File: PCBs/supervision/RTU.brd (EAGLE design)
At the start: 75 x 59 mm, 18 parts, among them IC1 LM1117T-1.8, IC2 7805T, M1 WIRELESS-NRF24L01, Q1 BC548, U1 ESP-WROOM-32, U2 MICROSD_CATALEX, U3 DS1307Z, Y2 32kHz

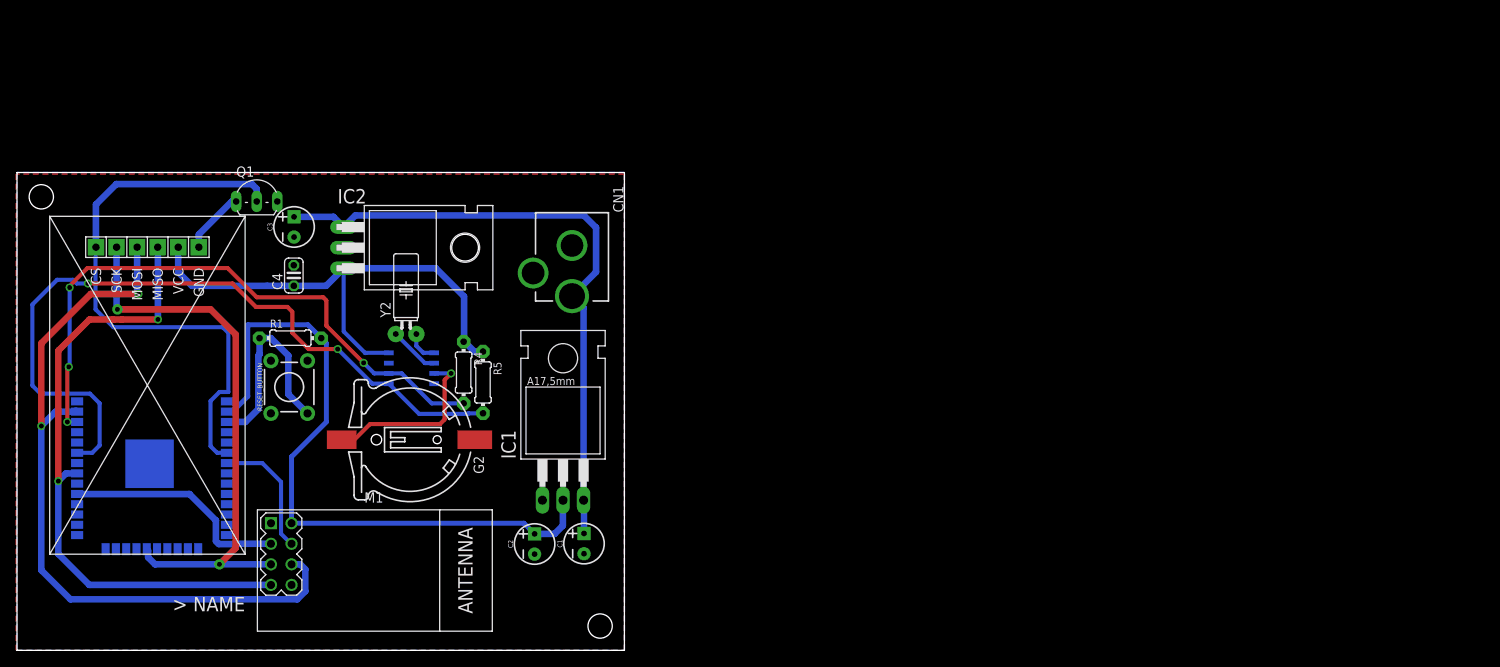
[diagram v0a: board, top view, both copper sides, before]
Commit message: Re-prototipação da PCB do sistema supervisorio
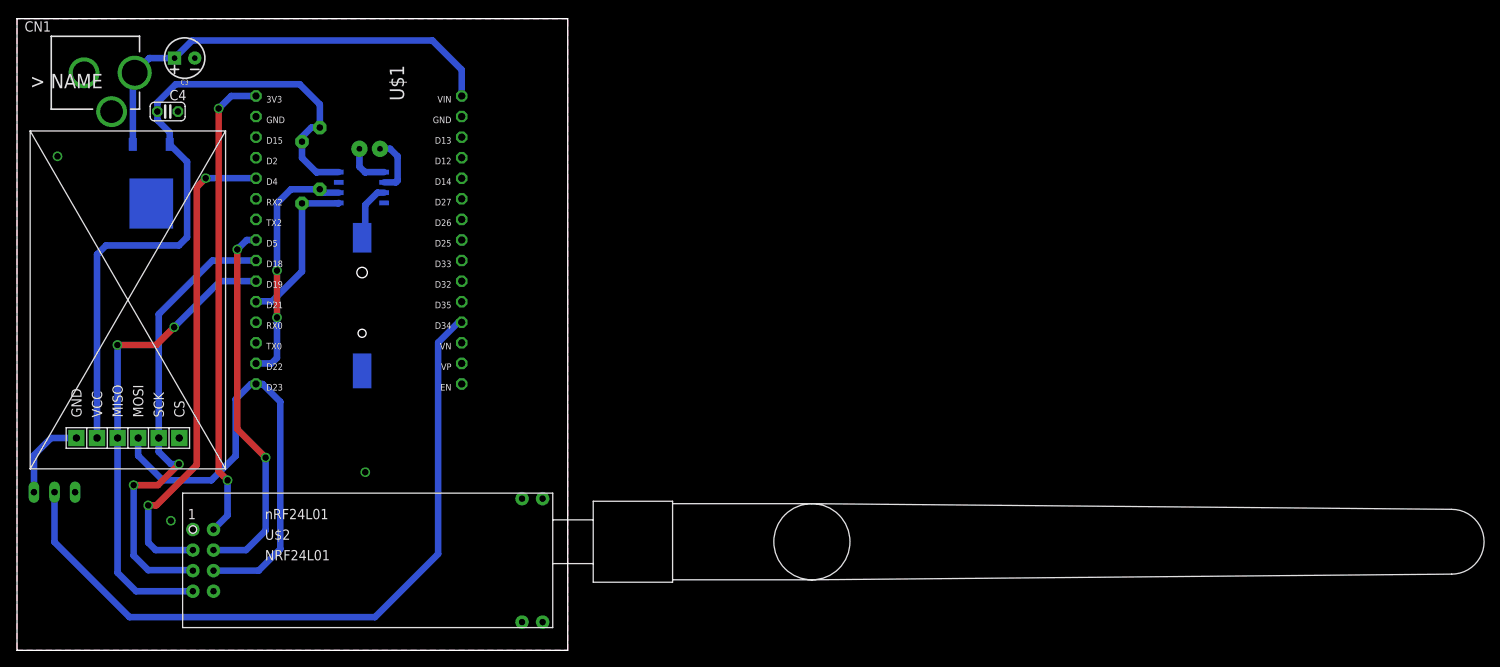
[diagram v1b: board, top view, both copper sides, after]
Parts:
- removed C1, C2: 10uF, SparkFun-Capacitors:CPOL-RADIAL-2.5MM-5MM
- removed IC1: LM1117T-1.8, lm1117:TO220
- removed M1: WIRELESS-NRF24L01, diy-modules:WIRELESS-NRF24L01
- removed R1: 10K, adafruit:0204/7
- removed RESET_BUTTON: MOMENTARY-SWITCH-SPST-PTH-6.0MM, SparkFun-Switches:TACTILE_SWITCH_PTH_6.0MM
- removed U1: ESP-WROOM-32, esp32:ESP-WROOM-32
- added U$1: ESP32_DEVKIT, DOIT_ESP32_DEVKIT:ESP32_DEVKIT
- added U$2: NRF24L01, Clean-Kong:NRF24L01
- IC2: value 7805T -> 7805DT; device linear:TO220H -> linear:TO252
- moved CN1 69.0 mm to (0.93, 71.3), turned to 270 degrees
- moved Q1 45.8 mm to (4.63, 18.3), flipped to the bottom, turned to 180 degrees
- moved U2 41.1 mm to (1.69, 22.3), turned to 0 degrees
- moved IC2 34.8 mm to (16.6, 57.7), flipped to the bottom, turned to 180 degrees
- moved R5 34.2 mm to (35.2, 59.0), flipped to the bottom
- moved R4 31.9 mm to (37.4, 60.7), flipped to the bottom
- moved C4 25.5 mm to (18.6, 66.5), turned to 0 degrees
- moved C3 24.8 mm to (20.7, 73.1), turned to 180 degrees
- moved Y2 23.3 mm to (43.5, 61.9), flipped to the bottom
- moved U3 23.2 mm to (42.5, 57.1)
- moved G2 22.6 mm to (42.6, 48.6), flipped to the bottom, turned to 180 degrees
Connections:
- removed net 3.3V: C2.1, IC1.2, M1.2, R1.2, U1.2
- removed net RESET: R1.1, RESET_BUTTON.3, U1.3
- new net 3V3: U$1.3V3, U$2.VCC
- new net USD: Q1.B, U$1.D34
- net 5V: now also IC2.2; no longer IC2.3
- net CE: now also U$1.D4, U$2.CE; no longer M1.3, U1.29
- net CS: no longer Q1.B, U1.6
- net CSN: now also U$1.D5, U$2.CSN; no longer M1.4, U1.7
- net GND: now also IC2.3, U$1.GND@1, U$1.GND@2, U$2.GND; no longer C1.2, C2.2, IC1.1, IC2.2, M1.1, RESET_BUTTON.1, U1.1, U1.15, U1.38, U1.GND
- net MISO: now also U$1.D19, U$2.MISO; no longer M1.7, U1.31
- net MOSI: now also U$1.D23, U$2.MOSI; no longer M1.6, U1.37
- net PWR: now also U$1.VIN; no longer C1.1, IC1.3
- net SCK: now also U$1.D18, U$2.SCK; no longer M1.5, U1.20
- net SCL: now also U$1.D22; no longer U1.36
- net SDA: now also U$1.D21; no longer U1.33
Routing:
- net USD: track 0.00 -> 90.7 mm
- net 3.3V: track 84.5 -> 0.00 mm
- net SDA: track 92.9 -> 20.2 mm, vias 2 -> 0
- net CS: track 71.2 -> 0.00 mm
- net 3V3: track 0.00 -> 58.4 mm, vias 0 -> 2
- net SCL: track 76.4 -> 30.5 mm, vias 4 -> 2
- net MOSI: track 92.9 -> 58.5 mm, vias 2 -> 0
- net CE: track 28.0 -> 60.6 mm, vias 0 -> 2
- net CSN: track 15.9 -> 46.4 mm, vias 0 -> 2
- net RESET: track 25.9 -> 0.00 mm
- net 5V: track 64.4 -> 88.3 mm
- net PWR: track 78.6 -> 55.7 mm
- net MISO: track 78.5 -> 58.8 mm
- net N$3: track 21.9 -> 7.17 mm, vias 1 -> 0
- net SCK: track 69.4 -> 58.3 mm
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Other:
- board size 75 x 59 mm -> 68 x 78 mm
